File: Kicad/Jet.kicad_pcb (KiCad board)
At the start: 2 copper layers, 17 parts, among them J1 Conn_02x13_Odd_Even, J2 Conn_01x03_Female, J3 POWER, J4 Conn_02x10_Odd_Even, J5 Conn_02x10_Odd_Even, Q1 BCW66FR, Q2 BCW66FR, U1 PC817, U2 PC817

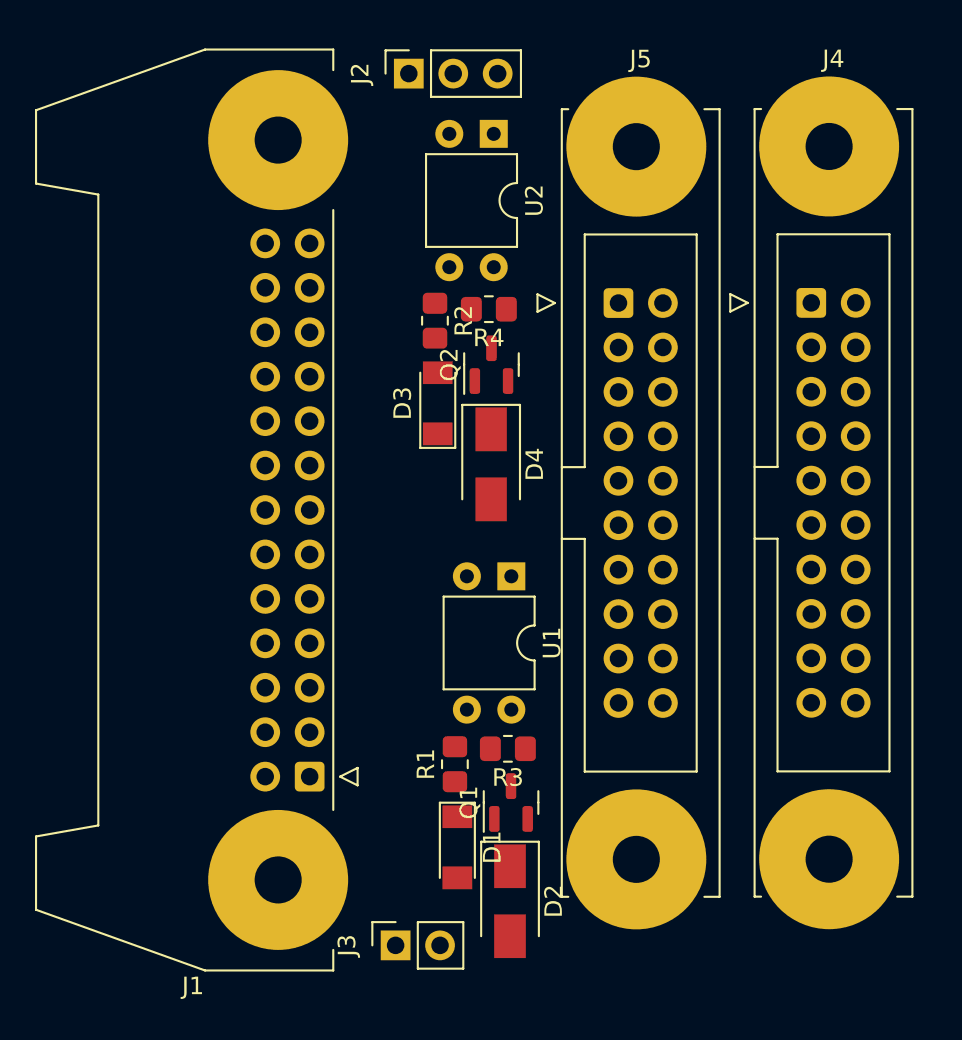
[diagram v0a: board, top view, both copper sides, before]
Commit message: FIX PCB
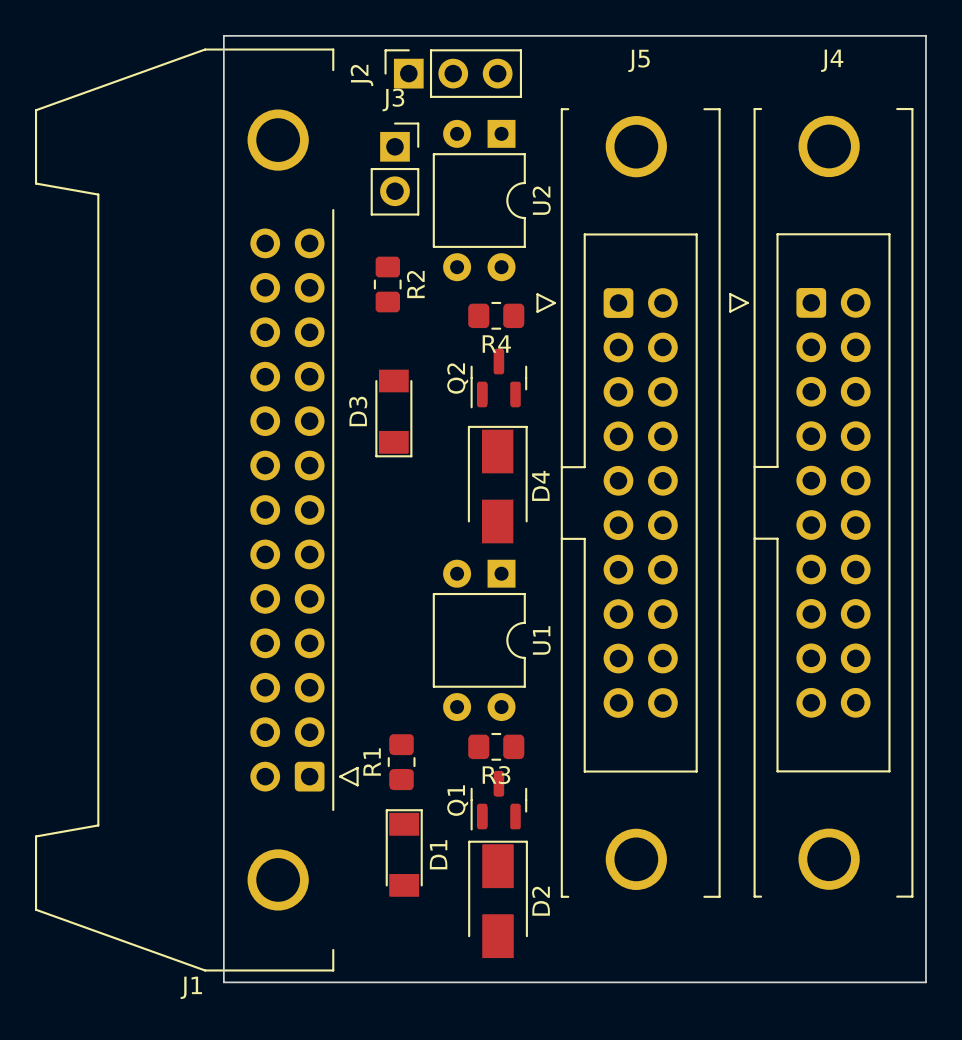
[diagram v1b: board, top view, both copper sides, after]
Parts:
- moved J3 45.6 mm to (101.5, 69.1), turned to 0 degrees
- moved R2 3.40 mm to (101.1, 77.0)
- moved D1 3.07 mm to (102.0, 109.5)
- moved R1 3.05 mm to (101.9, 104.2)
- moved D3 2.56 mm to (101.4, 84.2)
- moved D4 1.32 mm to (107.3, 88.5)
- moved Q2 0.88 mm to (107.4, 82.3)
- moved Q1 0.71 mm to (107.4, 106.4)
- moved D2 0.69 mm to (107.4, 112.2)
- moved R3 0.67 mm to (107.3, 103.4)
- moved U1 0.58 mm to (107.6, 93.5)
- moved R4 0.57 mm to (107.3, 78.7)
- moved U2 0.44 mm to (107.6, 68.3)
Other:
- board outline added: 40.1 x 54.1 mm
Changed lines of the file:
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@@
   (net 53 "Net-(R2-Pad1)")
   (footprint "Resistor_SMD:R_0805_2012Metric_Pad1.20x1.40mm_HandSolder" (layer "F.Cu")
-    (at 106.84 78.36 180)
+    (at 107.265 78.74 180)
     (descr "Resistor SMD 0805 (2012 Metric), square (rectangular) end terminal, IPC_7351 nominal with elongated pad for handsoldering. (Body size source: IPC-SM-782 page 72, https://www.pcb-3d.com/wordpress/wp-content/uploads/ipc-sm-782a_amendment_1_and_2.pdf), generated with kicad-footprint-generator")
     (tags "resistor handsolder")
@@
   )
   (footprint "Diode_SMD:D_SMA" (layer "F.Cu")
-    (at 108.05 112.2 -90)
+    (at 107.365 112.2 -90)
     (descr "Diode SMA (DO-214AC)")
     (tags "Diode SMA (DO-214AC)")
@@
   )
   (footprint "Diode_SMD:D_MiniMELF" (layer "F.Cu")
-    (at 103.92 83.74 90)
+    (at 101.41 84.22 90)
     (descr "Diode Mini-MELF (SOD-80)")
     (tags "Diode Mini-MELF (SOD-80)")
@@
     (pad "20" thru_hole circle (at 2.54 22.86) (size 1.7 1.7) (drill 1) (layers *.Cu *.Mask)
       (net 2 "GND") (pinfunction "Pin_20") (pintype "passive"))
-    (pad "MP" thru_hole circle (at 1.02 -8.94) (size 8 8) (drill 2.69) (layers *.Cu *.Mask))
-    (pad "MP" thru_hole circle (at 1.02 31.8) (size 8 8) (drill 2.69) (layers *.Cu *.Mask))
+    (pad "MP" thru_hole circle (at 1.02 -8.94) (size 3.5 3.5) (drill 2.5) (layers *.Cu *.Mask))
+    (pad "MP" thru_hole circle (at 1.02 31.8) (size 3.5 3.5) (drill 2.5) (layers *.Cu *.Mask))
     (model "${KICAD6_3DMODEL_DIR}/Connector_IDC.3dshapes/IDC-Header_2x10-1MP_P2.54mm_Latch_Vertical.wrl"
       (offset (xyz 0 0 0))
@@
   )
   (footprint "Resistor_SMD:R_0805_2012Metric_Pad1.20x1.40mm_HandSolder" (layer "F.Cu")
-    (at 104.9 104.37 90)
+    (at 101.854 104.25 90)
     (descr "Resistor SMD 0805 (2012 Metric), square (rectangular) end terminal, IPC_7351 nominal with elongated pad for handsoldering. (Body size source: IPC-SM-782 page 72, https://www.pcb-3d.com/wordpress/wp-content/uploads/ipc-sm-782a_amendment_1_and_2.pdf), generated with kicad-footprint-generator")
     (tags "resistor handsolder")
@@
   )
   (footprint "Package_DIP:DIP-4_W7.62mm" (layer "F.Cu")
-    (at 108.125 93.63 -90)
+    (at 107.565 93.482 -90)
     (descr "4-lead though-hole mounted DIP package, row spacing 7.62 mm (300 mils)")
     (tags "THT DIP DIL PDIP 2.54mm 7.62mm 300mil")
@@
   )
   (footprint "Resistor_SMD:R_0805_2012Metric_Pad1.20x1.40mm_HandSolder" (layer "F.Cu")
-    (at 107.93 103.49 180)
+    (at 107.265 103.378 180)
     (descr "Resistor SMD 0805 (2012 Metric), square (rectangular) end terminal, IPC_7351 nominal with elongated pad for handsoldering. (Body size source: IPC-SM-782 page 72, https://www.pcb-3d.com/wordpress/wp-content/uploads/ipc-sm-782a_amendment_1_and_2.pdf), generated with kicad-footprint-generator")
     (tags "resistor handsolder")
@@
   )
   (footprint "Package_DIP:DIP-4_W7.62mm" (layer "F.Cu")
-    (at 107.12 68.34 -90)
+    (at 107.565 68.34 -90)
     (descr "4-lead though-hole mounted DIP package, row spacing 7.62 mm (300 mils)")
     (tags "THT DIP DIL PDIP 2.54mm 7.62mm 300mil")
@@
     (pad "26" thru_hole circle (at 2.54 30.48 180) (size 1.7 1.7) (drill 1) (layers *.Cu *.Mask)
       (net 30 "IN_OBUDOWA") (pinfunction "Pin_26") (pintype "passive"))
-    (pad "MP" thru_hole circle (at 1.8 -5.905 180) (size 8 8) (drill 2.69) (layers *.Cu *.Mask))
-    (pad "MP" thru_hole circle (at 1.8 36.385 180) (size 8 8) (drill 2.69) (layers *.Cu *.Mask))
+    (pad "MP" thru_hole circle (at 1.8 -5.905 180) (size 3.5 3.5) (drill 2.5) (layers *.Cu *.Mask))
+    (pad "MP" thru_hole circle (at 1.8 36.385 180) (size 3.5 3.5) (drill 2.5) (layers *.Cu *.Mask))
     (model "${KICAD6_3DMODEL_DIR}/Connector_IDC.3dshapes/IDC-Header_2x13-1MP_P2.54mm_Latch_Horizontal.wrl"
       (offset (xyz 0 0 0))
@@
   )
   (footprint "Package_TO_SOT_SMD:SOT-23" (layer "F.Cu")
-    (at 108.11 106.56 90)
+    (at 107.415 106.426 90)
     (descr "SOT, 3 Pin (https://www.jedec.org/system/files/docs/to-236h.pdf variant AB), generated with kicad-footprint-generator ipc_gullwing_generator.py")
     (tags "SOT TO_SOT_SMD")
@@
   )
   (footprint "Package_TO_SOT_SMD:SOT-23" (layer "F.Cu")
-    (at 106.99 81.53 90)
+    (at 107.415 82.296 90)
     (descr "SOT, 3 Pin (https://www.jedec.org/system/files/docs/to-236h.pdf variant AB), generated with kicad-footprint-generator ipc_gullwing_generator.py")
     (tags "SOT TO_SOT_SMD")
@@
     (pad "20" thru_hole circle (at 2.54 22.86) (size 1.7 1.7) (drill 1) (layers *.Cu *.Mask)
       (net 2 "GND") (pinfunction "Pin_20") (pintype "passive"))
-    (pad "MP" thru_hole circle (at 1.02 -8.94) (size 8 8) (drill 2.69) (layers *.Cu *.Mask))
-    (pad "MP" thru_hole circle (at 1.02 31.8) (size 8 8) (drill 2.69) (layers *.Cu *.Mask))
+    (pad "MP" thru_hole circle (at 1.02 -8.94) (size 3.5 3.5) (drill 2.5) (layers *.Cu *.Mask))
+    (pad "MP" thru_hole circle (at 1.02 31.8) (size 3.5 3.5) (drill 2.5) (layers *.Cu *.Mask))
     (model "${KICAD6_3DMODEL_DIR}/Connector_IDC.3dshapes/IDC-Header_2x10-1MP_P2.54mm_Latch_Vertical.wrl"
       (offset (xyz 0 0 0))
@@
   )
   (footprint "Connector_PinSocket_2.54mm:PinSocket_1x02_P2.54mm_Vertical" (layer "F.Cu")
-    (at 101.51 114.725 90)
+    (at 101.475 69.08)
     (descr "Through hole straight socket strip, 1x02, 2.54mm pitch, single row (from Kicad 4.0.7), script generated")
     (tags "Through hole socket strip THT 1x02 2.54mm single row")
@@
     (property "Sheetname" "")
     (attr through_hole)
-    (fp_text reference "J3" (at 0 -2.77 90) (layer "F.SilkS")
-      (effects (font (size 1 1) (thickness 0.15)))
-    )
-    (fp_text value "POWER" (at 0 5.31 90) (layer "F.Fab")
-      (effects (font (size 1 1) (thickness 0.15)))
-    )
-    (fp_text user "${REFERENCE}" (at 0 1.27) (layer "F.Fab")
+    (fp_text reference "J3" (at 0 -2.77) (layer "F.SilkS")
+      (effects (font (size 1 1) (thickness 0.15)))
+    )
+    (fp_text value "POWER" (at 0 5.31) (layer "F.Fab")
+      (effects (font (size 1 1) (thickness 0.15)))
+    )
+    (fp_text user "${REFERENCE}" (at 0 1.27 90) (layer "F.Fab")
       (effects (font (size 1 1) (thickness 0.15)))
     )
@@
     (fp_line (start 1.27 3.81) (end -1.27 3.81) (layer "F.Fab") (width 0.1))
     (fp_line (start -1.27 3.81) (end -1.27 -1.27) (layer "F.Fab") (width 0.1))
-    (pad "1" thru_hole rect (at 0 0 90) (size 1.7 1.7) (drill 1) (layers *.Cu *.Mask)
+    (pad "1" thru_hole rect (at 0 0) (size 1.7 1.7) (drill 1) (layers *.Cu *.Mask)
       (net 7 "VCC") (pinfunction "Pin_1") (pintype "passive"))
-    (pad "2" thru_hole oval (at 0 2.54 90) (size 1.7 1.7) (drill 1) (layers *.Cu *.Mask)
+    (pad "2" thru_hole oval (at 0 2.54) (size 1.7 1.7) (drill 1) (layers *.Cu *.Mask)
       (net 2 "GND") (pinfunction "Pin_2") (pintype "passive"))
     (model "${KICAD6_3DMODEL_DIR}/Connector_PinSocket_2.54mm.3dshapes/PinSocket_1x02_P2.54mm_Vertical.wrl"
@@
   )
   (footprint "Diode_SMD:D_MiniMELF" (layer "F.Cu")
-    (at 105.04 109.12 -90)
+    (at 102.004 109.55 -90)
     (descr "Diode Mini-MELF (SOD-80)")
     (tags "Diode Mini-MELF (SOD-80)")
@@
   )
   (footprint "Diode_SMD:D_SMA" (layer "F.Cu")
-    (at 106.97 87.23 -90)
+    (at 107.35 88.49 -90)
     (descr "Diode SMA (DO-214AC)")
     (tags "Diode SMA (DO-214AC)")
@@
   )
   (footprint "Resistor_SMD:R_0805_2012Metric_Pad1.20x1.40mm_HandSolder" (layer "F.Cu")
-    (at 103.76 79.02 -90)
+    (at 101.06 76.95 -90)
     (descr "Resistor SMD 0805 (2012 Metric), square (rectangular) end terminal, IPC_7351 nominal with elongated pad for handsoldering. (Body size source: IPC-SM-782 page 72, https://www.pcb-3d.com/wordpress/wp-content/uploads/ipc-sm-782a_amendment_1_and_2.pdf), generated with kicad-footprint-generator")
     (tags "resistor handsolder")
@@
     )
   )
+  (gr_rect (start 91.694 62.738) (end 131.826 116.84) (layer "Edge.Cuts") (width 0.1) (fill none))
 )

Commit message: FIX PCB
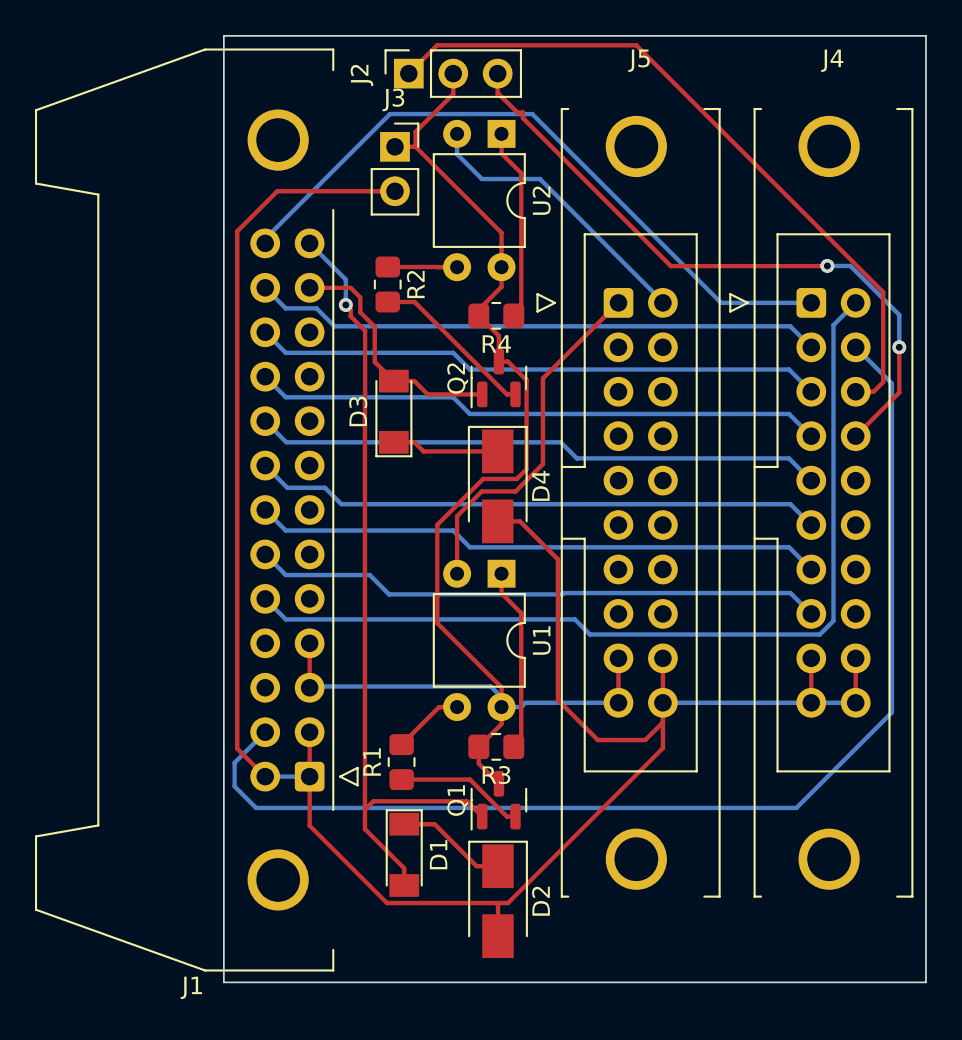
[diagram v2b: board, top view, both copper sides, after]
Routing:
- net GND: track 0.00 -> 119.4 mm
- net VCC: track 0.00 -> 76.4 mm
- net IN_AGREGAT_RESET: track 0.00 -> 65.9 mm
- net IN_AGREGAT_REKA: track 0.00 -> 52.4 mm
- net KOLO: track 0.00 -> 46.2 mm, vias 0 -> 1
- net TIME+: track 0.00 -> 40.6 mm
- net IN_OBUDOWA: track 0.00 -> 38.9 mm
- net TIME-: track 0.00 -> 37.5 mm, vias 0 -> 2
- net IN_WANNA: track 0.00 -> 32.7 mm
- net IN_START: track 0.00 -> 32.6 mm
- net IN_AGREGAT_KRANCOWKA: track 0.00 -> 32.6 mm
- net IN_CONFIG2: track 0.00 -> 32.6 mm
- net IN_KOLO_KRANCOWKA: track 0.00 -> 32.6 mm
- net IN_INTERWAL: track 0.00 -> 32.6 mm
- net IN_CONFIG1: track 0.00 -> 32.6 mm
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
